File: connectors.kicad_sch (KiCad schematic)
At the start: 26 parts, among them J1 USB_C_Receptacle_USB2.0_16P, J2 USB_C_Receptacle_PowerOnly_6P, J3 Conn_01x02, J4 Conn_ARM_SWD_TagConnect_TC203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, U24 TMUX154ERSW, U5 FUSB302B10MPX, U6 FUSB302B11MPX, U9 FUSB302B01MPX

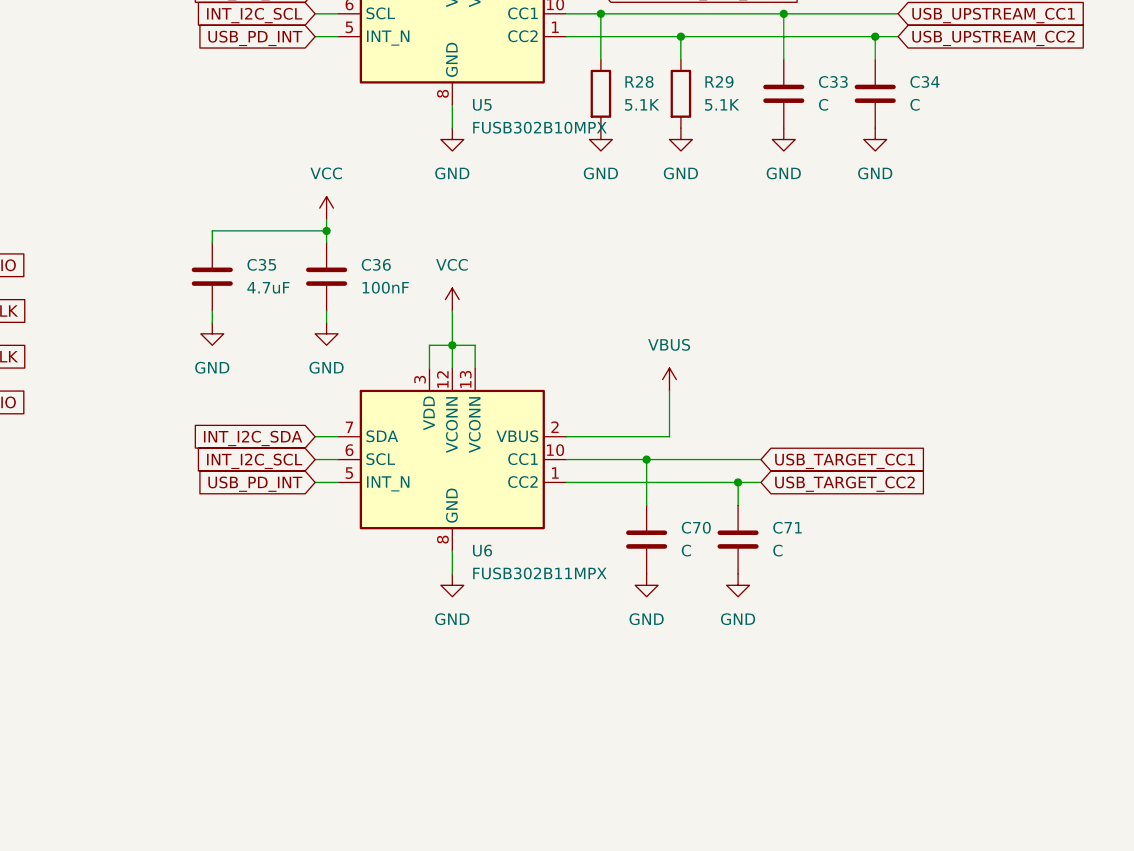
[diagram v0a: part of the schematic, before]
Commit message: Place elements
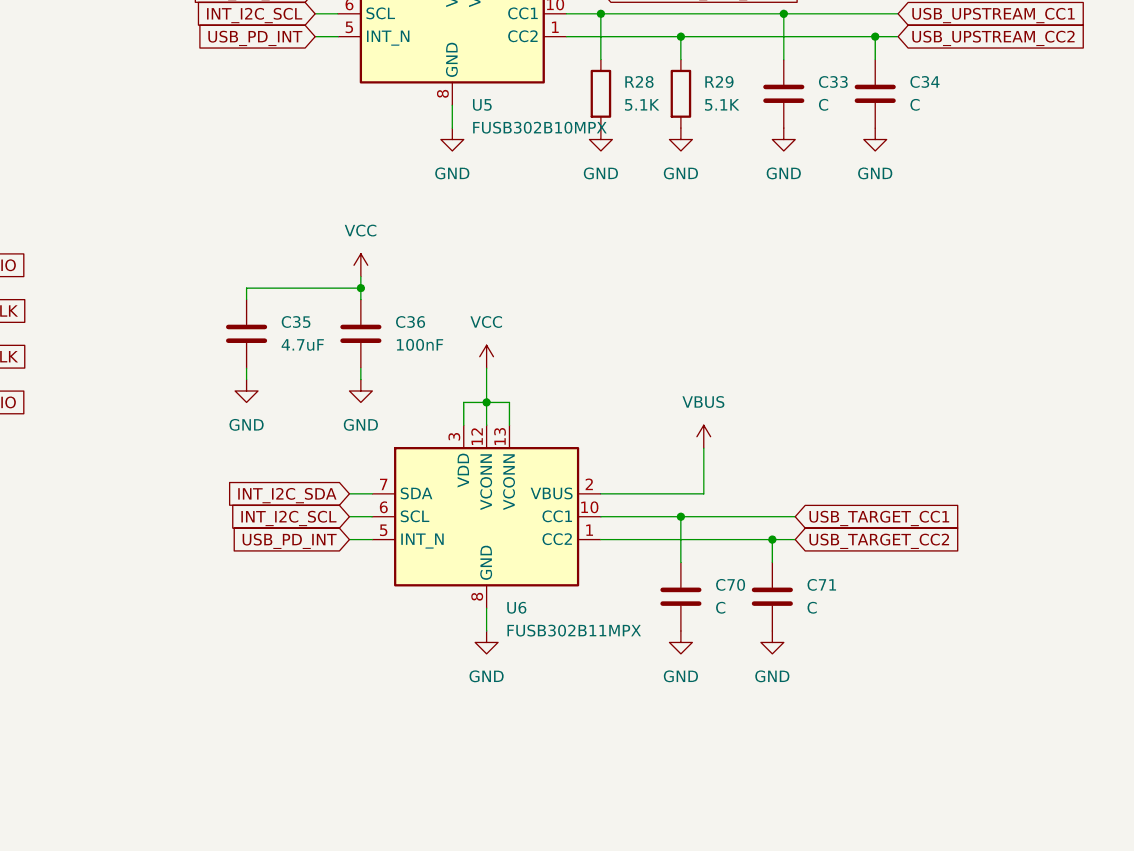
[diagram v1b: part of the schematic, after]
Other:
- moved on the sheet: C35, C36, C70, C71, U6
